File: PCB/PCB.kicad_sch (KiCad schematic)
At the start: 6 parts

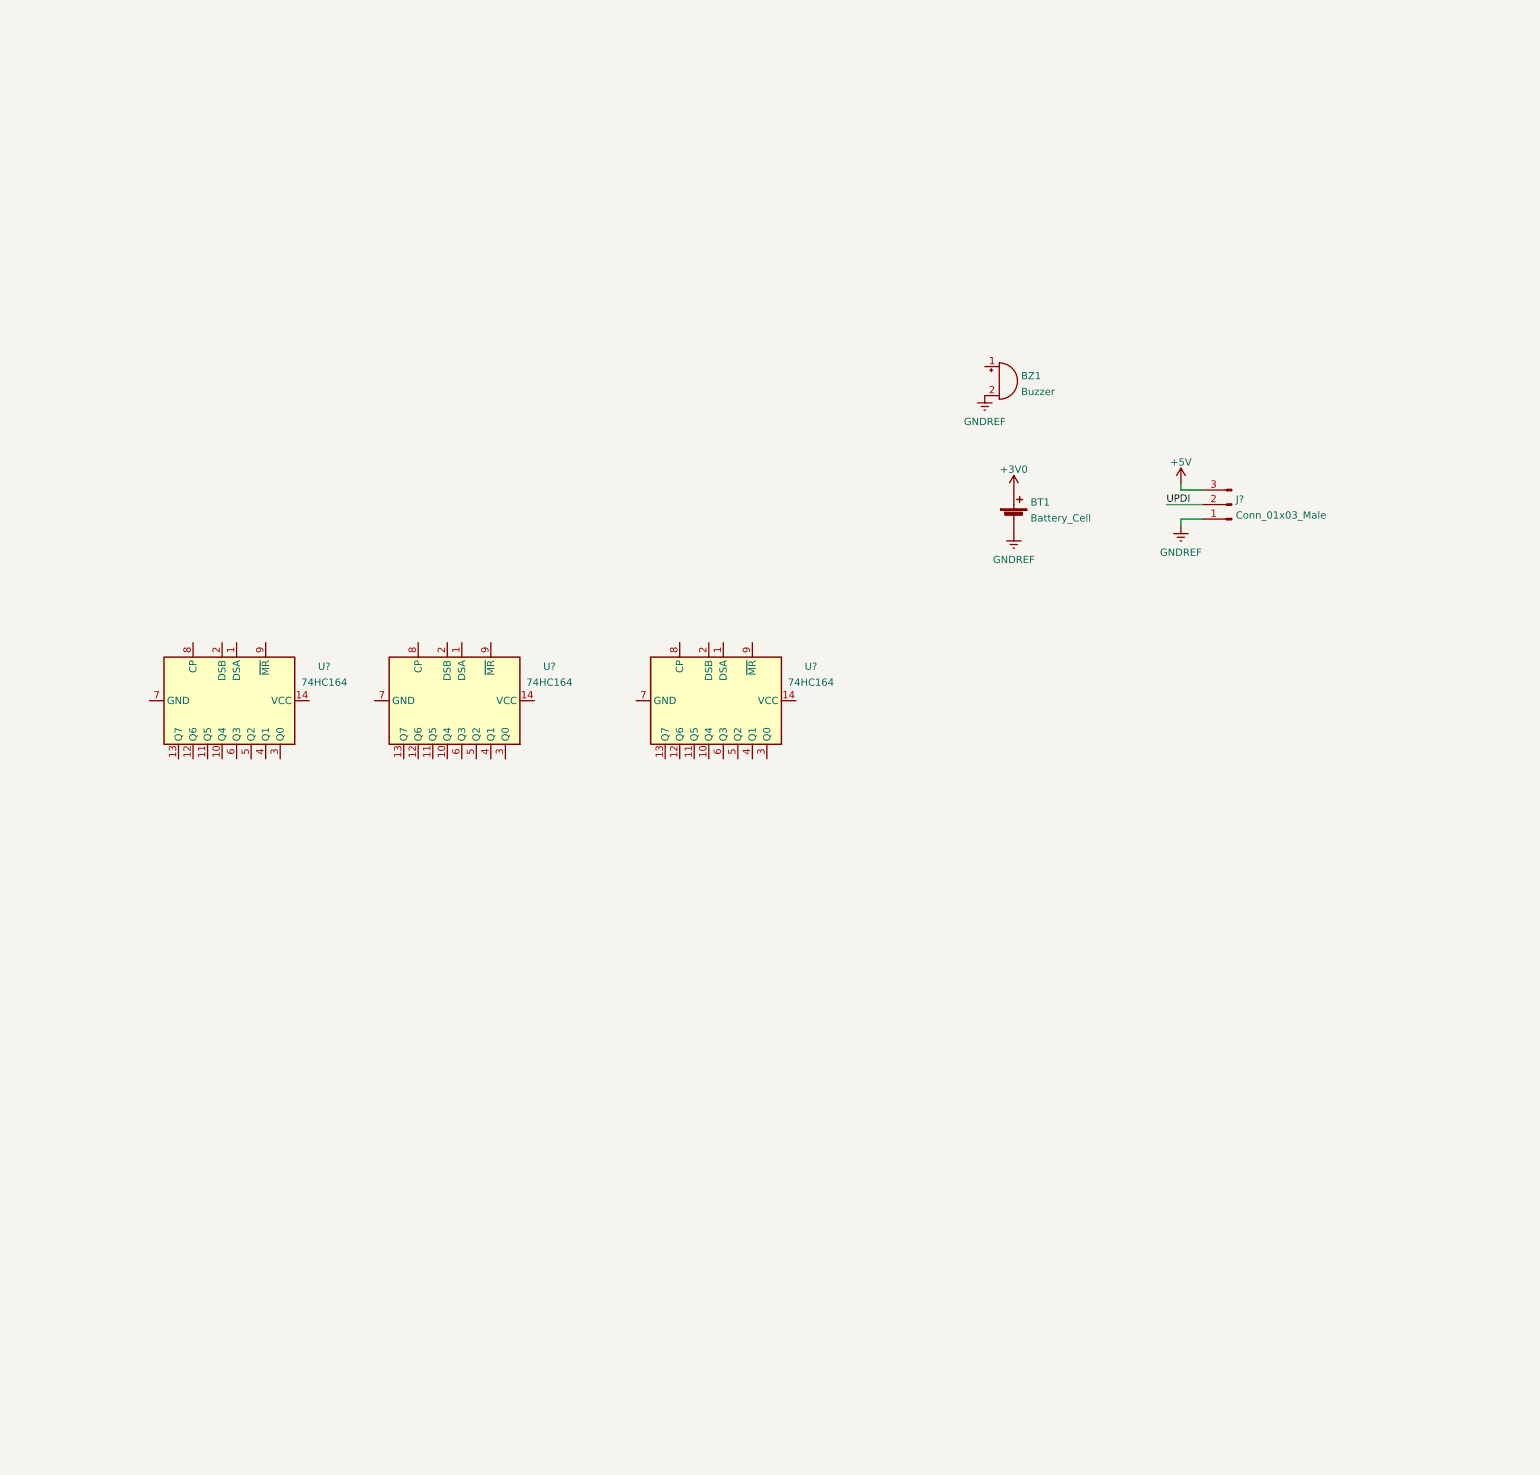
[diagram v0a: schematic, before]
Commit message: schematic almost done
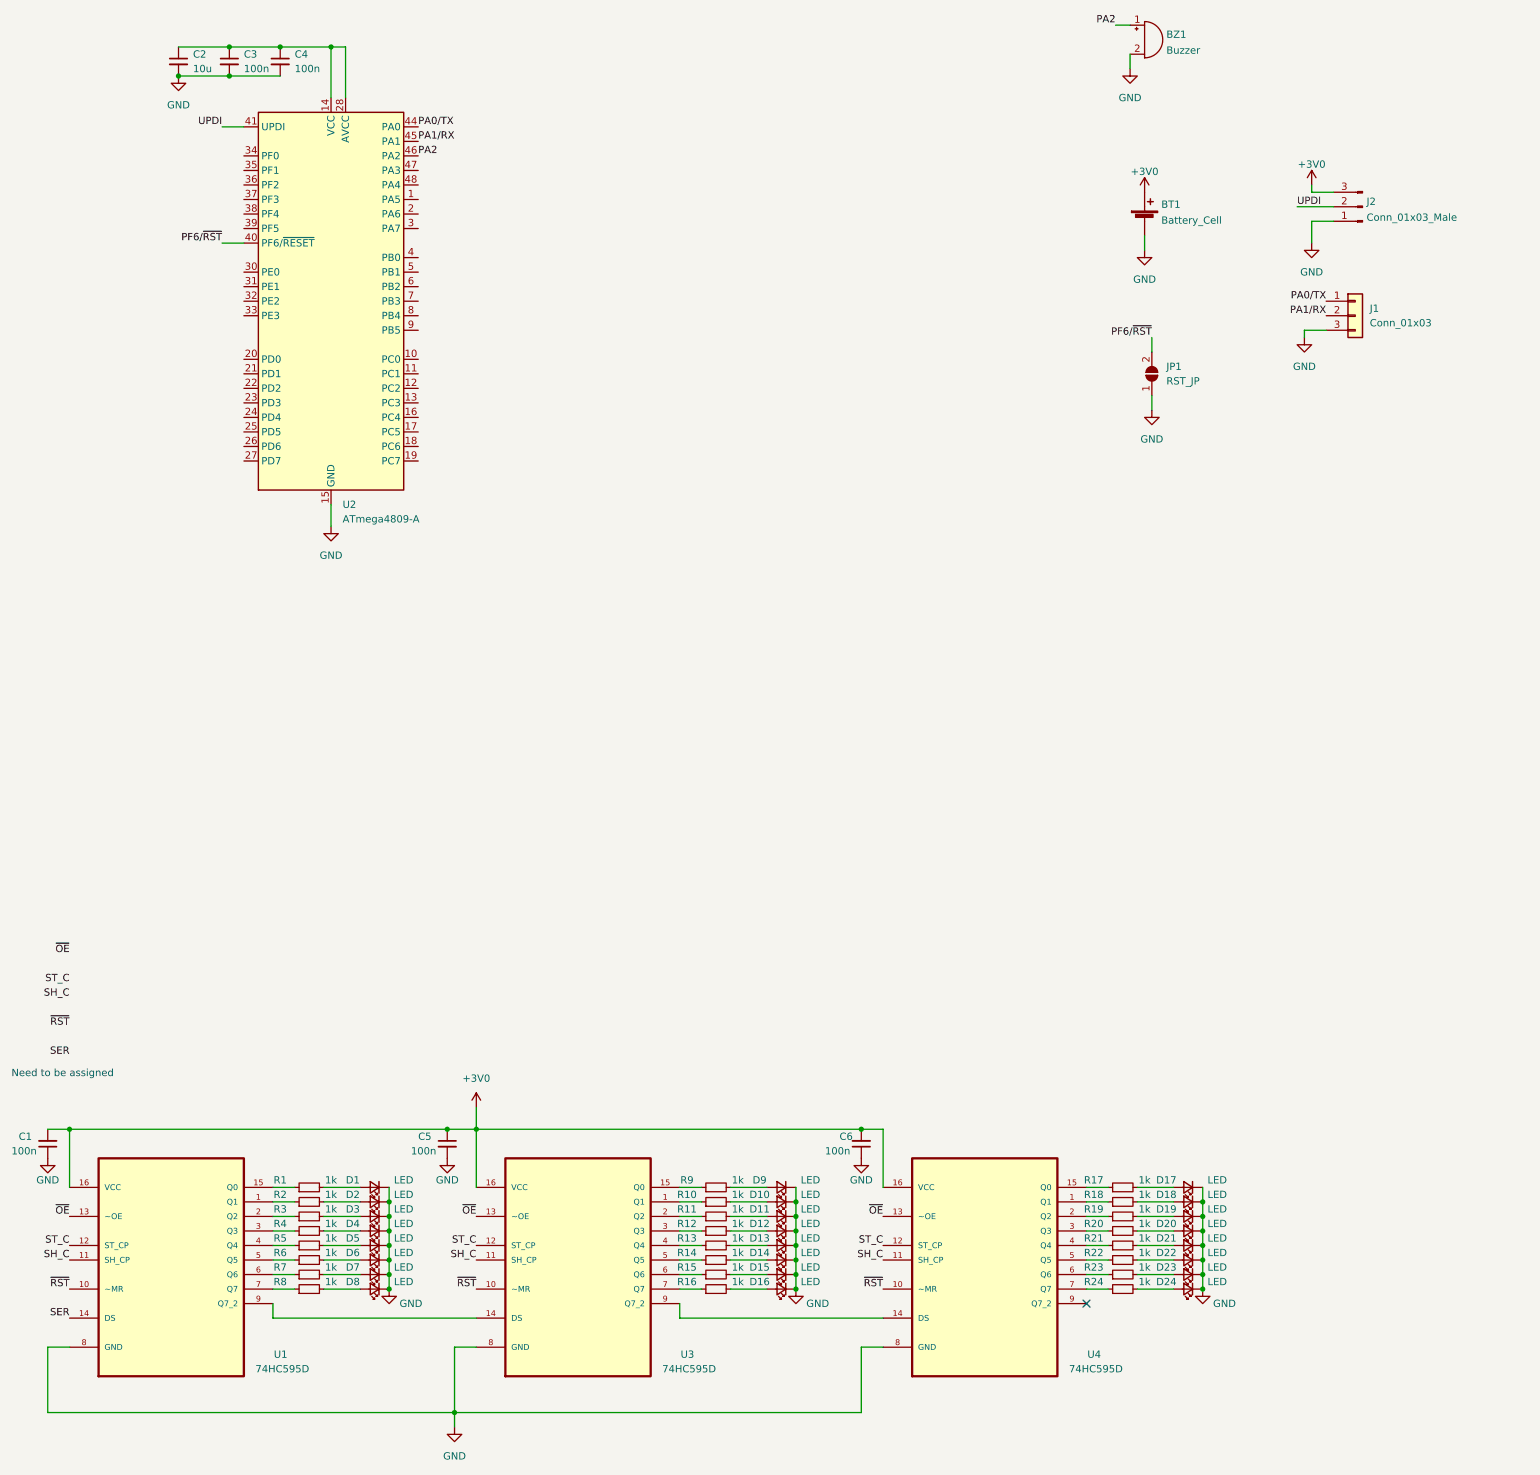
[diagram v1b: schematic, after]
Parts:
- removed U? (x3): 74HC164, Package_SO:SOIC-14_3.9x8.7mm_P1.27mm, symbol 74xx:74HC164
- added C1, C3, C4, C5, C6: 100n, Capacitor_SMD:C_0603_1608Metric, symbol Device:C_Small
- added C2: 10u, Capacitor_SMD:C_0603_1608Metric, symbol Device:C_Small
- added D1, D10, D11, D12, D13, D14, D15, D16, D17, D18, D19, D2, D20, D21, D22, D23, D24, D3, D4, D5, D6, D7, D8, D9: LED, LED_SMD:LED_0603_1608Metric, symbol Device:LED_Small
- added J1: Conn_01x03, Connector_PinHeader_2.54mm:PinHeader_1x03_P2.54mm_Vertical, symbol Connector_Generic:Conn_01x03
- added JP1: RST_JP, Jumper:SolderJumper-2_P1.3mm_Open_RoundedPad1.0x1.5mm, symbol Jumper:SolderJumper_2_Open
- added R1, R10, R11, R12, R13, R14, R15, R16, R17, R18, R19, R2, R20, R21, R22, R23, R24, R3, R4, R5, R6, R7, R8, R9: 1k, Resistor_SMD:R_0603_1608Metric, symbol Device:R_Small
- added U1, U3, U4: 74HC595D, xmasLib:SOIC127P600X175-16N, symbol 74HC595D_118:74HC595D,118
- added U2: ATmega4809-A, Package_QFP:TQFP-48_7x7mm_P0.5mm, symbol MCU_Microchip_ATmega:ATmega4809-A
- gave numbers to parts that had none: 1
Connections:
- net +5V is gone; now on net +3V0: J2.3 (Pin_3)
- net +3V0: now also C1.2, C5.1, C6.2, U1.16 (VCC), U3.16 (VCC), U4.16 (VCC)
- net UPDI: now also U2.41 (UPDI)
- net PA2: now reaches BZ1.1 (-)
- net PA2: now also U2.46 (PA2)
- net GNDREF renamed GND
- net GND: now also C1.1, C2.2, C3.2, C4.2, C5.2, C6.1, D1.1 (K), D10.1 (K), D11.1 (K), D12.1 (K), D13.1 (K), D14.1 (K), D15.1 (K), D16.1 (K), D17.1 (K), D18.1 (K), D19.1 (K), D2.1 (K), D20.1 (K), D21.1 (K), D22.1 (K), D23.1 (K), D24.1 (K), D3.1 (K), D4.1 (K), D5.1 (K), D6.1 (K), D7.1 (K), D8.1 (K), D9.1 (K), J1.3 (Pin_3), JP1.1 (A), U1.8 (GND), U2.15 (GND), U2.29 (GND), U2.43 (GND), U3.8 (GND), U4.8 (GND)
- new net: R6.1, U1.5 (Q5)
- new net: D6.2 (A), R6.2
- new net: R13.1, U3.4 (Q4)
- new net: D13.2 (A), R13.2
- new net: D9.2 (A), R9.2
- new net: R2.1, U1.1 (Q1)
- new net: R1.1, U1.15 (Q0)
- new net: R3.1, U1.2 (Q2)
- new net: R4.1, U1.3 (Q3)
- new net: R5.1, U1.4 (Q4)
- new net: R7.1, U1.6 (Q6)
- new net: R8.1, U1.7 (Q7)
- new net: U1.9 (Q7_2), U3.14 (DS)
- new net: R21.1, U4.4 (Q4)
- new net: D21.2 (A), R21.2
- new net: D2.2 (A), R2.2
- new net: D12.2 (A), R12.2
- new net: D5.2 (A), R5.2
- new net: D16.2 (A), R16.2
- new net: D8.2 (A), R8.2
- new net: C2.1, C3.1, C4.1, U2.14 (VCC), U2.28 (AVCC), U2.42 (VCC)
- new net: D3.2 (A), R3.2
- new net: R15.1, U3.6 (Q6)
- new net: D15.2 (A), R15.2
- new net: R10.1, U3.1 (Q1)
- new net: D10.2 (A), R10.2
- new net: D17.2 (A), R17.2
- new net: D4.2 (A), R4.2
- new net: R20.1, U4.3 (Q3)
- new net: D20.2 (A), R20.2
- new net: R9.1, U3.15 (Q0)
- new net: D19.2 (A), R19.2
- new net: D7.2 (A), R7.2
- new net: D18.2 (A), R18.2
- new net: R16.1, U3.7 (Q7)
- new net: R17.1, U4.15 (Q0)
- new net: R11.1, U3.2 (Q2)
- new net: R12.1, U3.3 (Q3)
- new net: R14.1, U3.5 (Q5)
- new net: U3.9 (Q7_2), U4.14 (DS)
- new net: R22.1, U4.5 (Q5)
- new net: D22.2 (A), R22.2
- new net: D11.2 (A), R11.2
- new net: R24.1, U4.7 (Q7)
- new net: D24.2 (A), R24.2
- new net: D1.2 (A), R1.2
- new net: D14.2 (A), R14.2
- new net: R23.1, U4.6 (Q6)
- new net: D23.2 (A), R23.2
- new net: R18.1, U4.1 (Q1)
- new net: R19.1, U4.2 (Q2)
- new net PA0/TX: J1.1 (Pin_1), U2.44 (PA0)
- new net PA1/RX: J1.2 (Pin_2), U2.45 (PA1)
- new net PF6/~{RST}: JP1.2 (B), U2.40 (PF6/~{RESET})
- new net SER: U1.14 (DS)
- new net SH_C: U1.11 (SH_CP), U3.11 (SH_CP), U4.11 (SH_CP)
- new net ST_C: U1.12 (ST_CP), U3.12 (ST_CP), U4.12 (ST_CP)
- new net ~{OE}: U1.13 (~OE), U3.13 (~OE), U4.13 (~OE)
- new net ~{RST}: U1.10 (~MR), U3.10 (~MR), U4.10 (~MR)
- no-connect marks 0 -> 1
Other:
- note added: "Need to be assigned"
- moved on the sheet: BT1, BZ1, J2

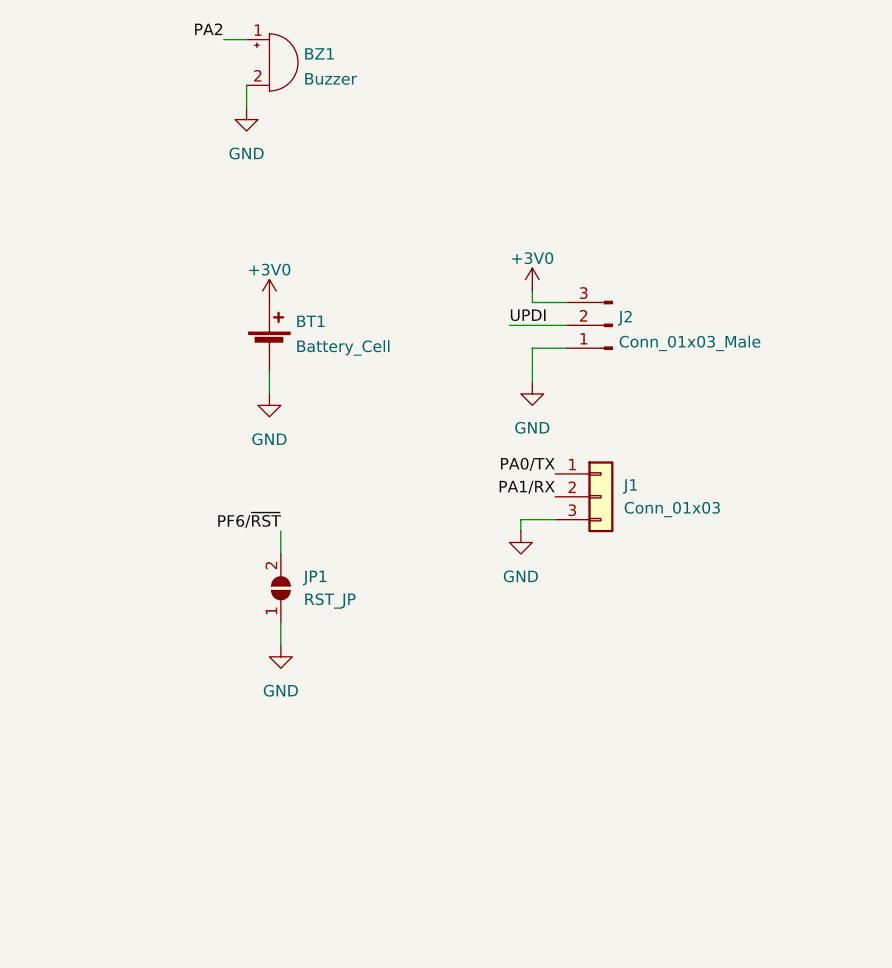
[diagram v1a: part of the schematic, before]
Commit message: Update PCB.kicad_sch
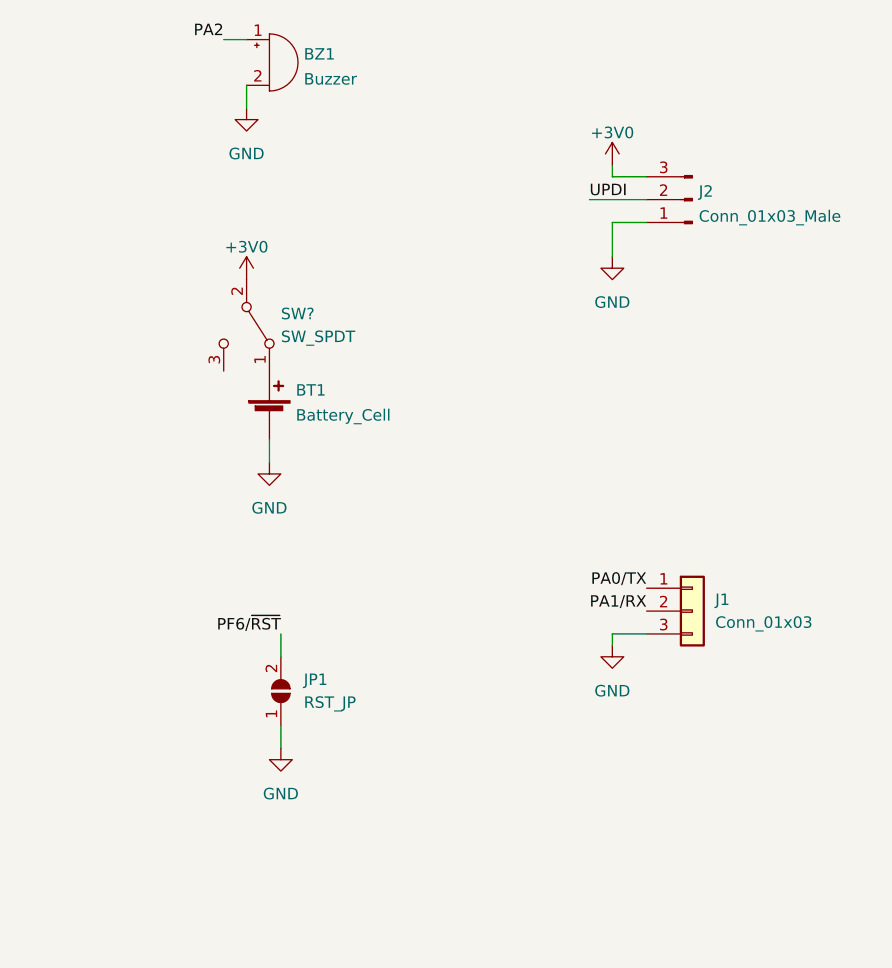
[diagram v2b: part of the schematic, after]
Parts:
- added SW?: SW_SPDT, symbol Switch:SW_SPDT
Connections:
- net +3V0: now also SW?.2 (B); no longer BT1.1 (+)
- new net: BT1.1 (+), SW?.1 (A)
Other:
- moved on the sheet: BT1, J1, J2, JP1
